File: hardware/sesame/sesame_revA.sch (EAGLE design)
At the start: 4 parts, among them Q1 TIP120

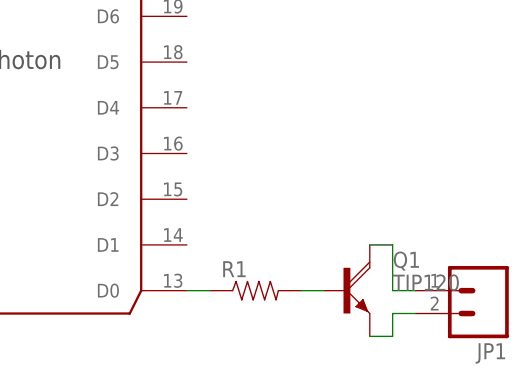
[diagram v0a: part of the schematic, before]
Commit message: fixing sesame
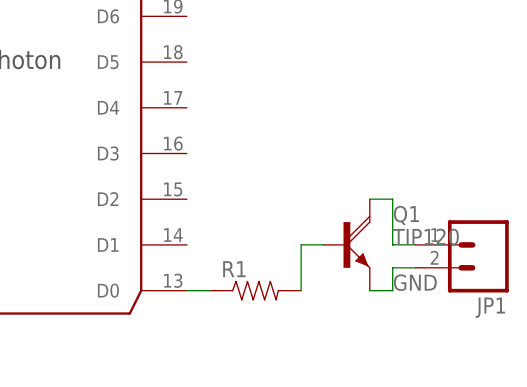
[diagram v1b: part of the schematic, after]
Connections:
- net N$2 renamed GND
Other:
- moved on the sheet: JP1, Q1
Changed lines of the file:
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@@
 <instances>
 <instance part="U$1" gate="G$1" x="33.02" y="53.34"/>
-<instance part="Q1" gate="1" x="68.58" y="25.4"/>
-<instance part="JP1" gate="G$1" x="83.82" y="25.4" rot="R180"/>
+<instance part="Q1" gate="1" x="68.58" y="30.48"/>
+<instance part="JP1" gate="G$1" x="83.82" y="30.48" rot="R180"/>
 <instance part="R1" gate="G$1" x="58.42" y="25.4"/>
 </instances>
@@
 <segment>
 <pinref part="Q1" gate="1" pin="C"/>
-<wire x1="71.12" y1="30.48" x2="73.66" y2="30.48" width="0.1524" layer="91"/>
-<wire x1="73.66" y1="30.48" x2="73.66" y2="25.4" width="0.1524" layer="91"/>
+<wire x1="71.12" y1="35.56" x2="73.66" y2="35.56" width="0.1524" layer="91"/>
+<wire x1="73.66" y1="35.56" x2="73.66" y2="30.48" width="0.1524" layer="91"/>
 <pinref part="JP1" gate="G$1" pin="1"/>
-<wire x1="73.66" y1="25.4" x2="76.2" y2="25.4" width="0.1524" layer="91"/>
+<wire x1="73.66" y1="30.48" x2="76.2" y2="30.48" width="0.1524" layer="91"/>
 </segment>
 </net>
-<net name="N$2" class="0">
+<net name="GND" class="0">
 <segment>
+<pinref part="Q1" gate="1" pin="E"/>
+<wire x1="73.66" y1="25.4" x2="71.12" y2="25.4" width="0.1524" layer="91"/>
 <pinref part="JP1" gate="G$1" pin="2"/>
-<wire x1="76.2" y1="22.86" x2="73.66" y2="22.86" width="0.1524" layer="91"/>
-<wire x1="73.66" y1="22.86" x2="73.66" y2="20.32" width="0.1524" layer="91"/>
-<pinref part="Q1" gate="1" pin="E"/>
-<wire x1="73.66" y1="20.32" x2="71.12" y2="20.32" width="0.1524" layer="91"/>
-</segment>
-</net>
-<net name="N$3" class="0">
-<segment>
-<pinref part="Q1" gate="1" pin="B"/>
-<pinref part="R1" gate="G$1" pin="2"/>
-<wire x1="63.5" y1="25.4" x2="66.04" y2="25.4" width="0.1524" layer="91"/>
+<wire x1="76.2" y1="27.94" x2="73.66" y2="27.94" width="0.1524" layer="91"/>
+<wire x1="73.66" y1="27.94" x2="73.66" y2="25.4" width="0.1524" layer="91"/>
+<label x="73.66" y="25.4" size="1.778" layer="95"/>
 </segment>
 </net>
@@
 </segment>
 </net>
+<net name="N$2" class="0">
+<segment>
+<pinref part="R1" gate="G$1" pin="2"/>
+<wire x1="63.5" y1="25.4" x2="63.5" y2="30.48" width="0.1524" layer="91"/>
+<pinref part="Q1" gate="1" pin="B"/>
+<wire x1="63.5" y1="30.48" x2="66.04" y2="30.48" width="0.1524" layer="91"/>
+</segment>
+</net>
